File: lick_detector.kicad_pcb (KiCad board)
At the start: 2 copper layers, 19 x 19 mm, 15 parts, among them P1 CONN_FFC_8_VERT, U1 ADXL313, U2 BUFFER_TRI_STATE_SMALL, U3 BUFFER_2_ELEMENT_SMALL

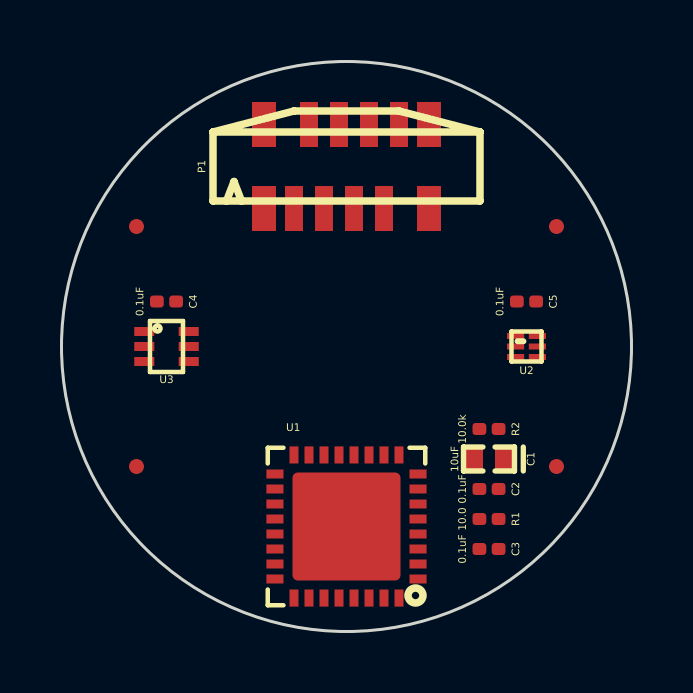
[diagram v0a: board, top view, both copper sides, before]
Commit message: Rectangular outline
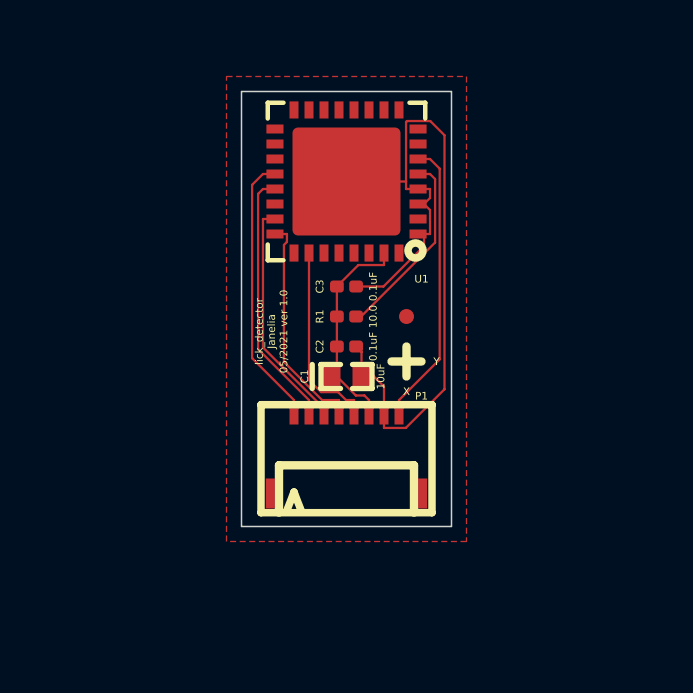
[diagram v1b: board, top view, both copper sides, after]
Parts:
- removed C4, C5: 0.1uF, lick_detector:SM0201
- removed FID2, FID3, FID4: FIDUCIAL, lick_detector:FIDUCIAL
- removed R2: 10.0k, lick_detector:SM0201
- removed U2: BUFFER_TRI_STATE_SMALL, lick_detector:MICROPAK2_6LEAD
- removed U3: BUFFER_2_ELEMENT_SMALL, lick_detector:SOT-563
- P1: value CONN_FFC_8_VERT -> CONN_FFC_8_RA; footprint lick_detector:Molex_FFC_1x8_P0.5mm_Vertical -> lick_detector:Molex_FFC_1x8_P0.5mm_RA
- moved U1 11.5 mm to (150.0, 94.5)
- moved C3 9.96 mm to (150.0, 98.0), turned to 0 degrees
- moved FID1 9.49 mm to (152.0, 99.0)
- moved R1 8.25 mm to (150.0, 99.0), turned to 0 degrees
- moved P1 8.25 mm to (150.0, 102.2)
- moved C2 6.72 mm to (150.0, 100.0), turned to 0 degrees
- moved C1 5.49 mm to (150.0, 101.0), turned to 90 degrees
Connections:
- P1 pad 1: GND -> /INT1
- P1 pad 2: /MOSI -> /INT2
- P1 pad 3: /INT1 -> /MISO
- P1 pad 4: /SCK -> /MOSI
- P1 pad 5: /INT2 -> /SCK
- P1 pad 6: /MISO -> VAA
- P1 pad 7: /~CS -> GND
- P1 pad 8: VAA -> /~CS
- U1 pad 20: /INT1_UB -> /INT1
- U1 pad 21: /INT2_UB -> /INT2
- U1 pad 23: /MISO_UB -> /MISO
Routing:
- net GND: track 0.00 -> 26.4 mm
- net /~CS: track 0.00 -> 9.59 mm
- net /INT1: track 0.00 -> 9.13 mm
- net /INT2: track 0.00 -> 8.67 mm
- net /MISO: track 0.00 -> 7.74 mm
- net /MOSI: track 0.00 -> 7.53 mm
- net VAA: track 0.00 -> 7.31 mm
- net /SCK: track 0.00 -> 6.47 mm
- net Net-(R1-Pad2): track 0.00 -> 6.41 mm
- added copper zone on F.Cu, net GND
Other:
- board size 19 x 19 mm -> 7 x 14.5 mm
- net class Default: trace_width 0.2032 -> 0.0762; via_dia 0.3048 -> 0.254
- net class POWER: trace_width 0.1524 -> 0.0762; via_dia 0.3048 -> 0.254
- net class SIGNAL: trace_width 0.1524 -> 0.0762; via_dia 0.3048 -> 0.254
- rule trace_min: 0.1016 -> 0.0762
- board text added: "X"
- board text added: "Y"
- board text added: "lick_detector Janelia 05/2021 ver 1.0"
- board text removed: "lick_detector Janelia Research Campus 04/2021 ver 1.0"

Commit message: Export supplementals
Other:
- rule pad_to_mask_clearance: 0.0508 -> 0
